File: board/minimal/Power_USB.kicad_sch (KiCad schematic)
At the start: 11 parts, among them J2 USB_C_Receptacle_USB2.0_14P, U4 STUSB4500QTR

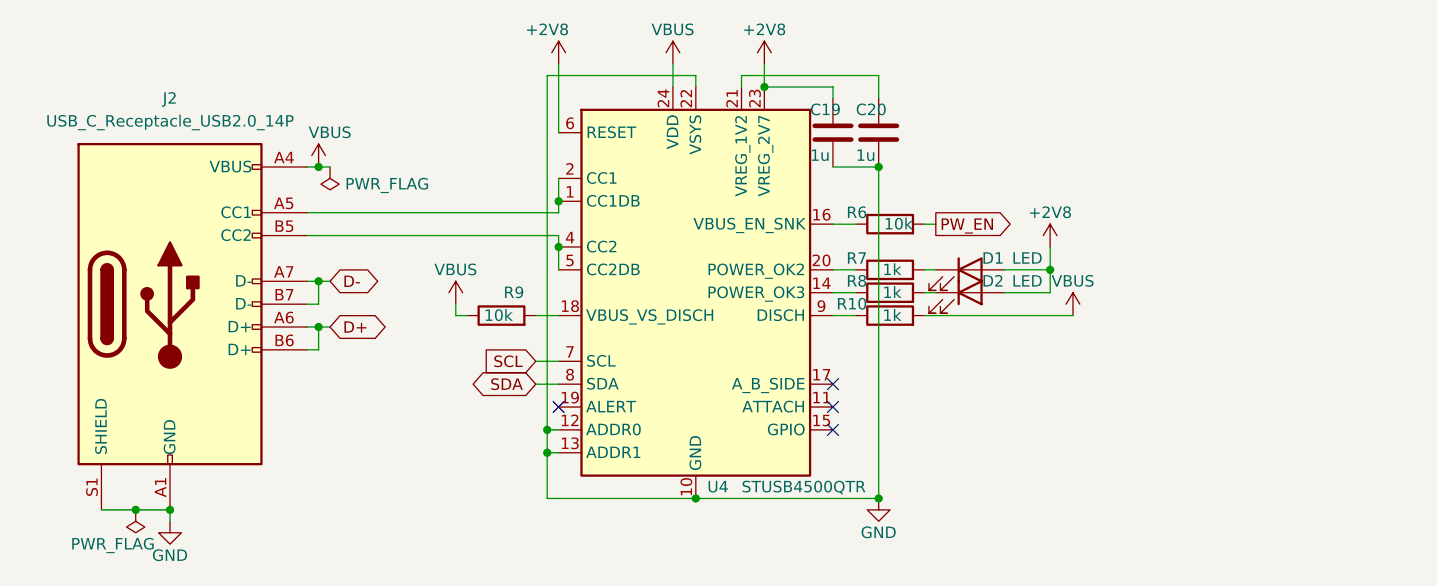
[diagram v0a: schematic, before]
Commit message: update PCB and edit schematic
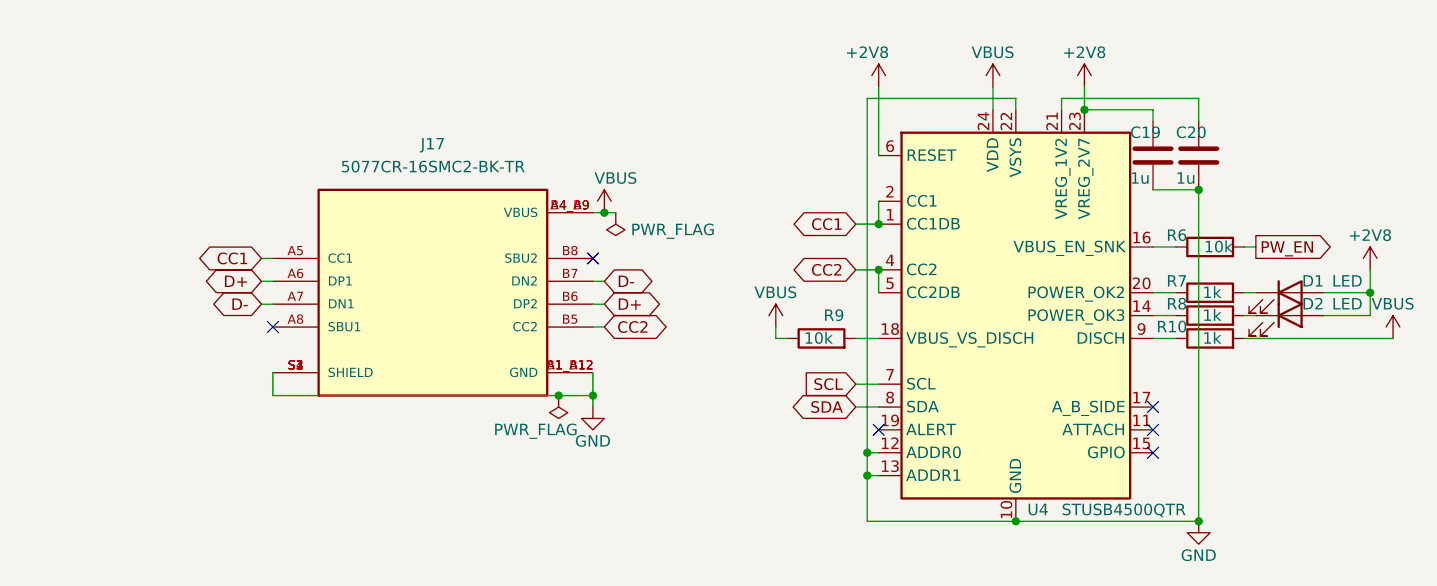
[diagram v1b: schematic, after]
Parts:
- removed J2: USB_C_Receptacle_USB2.0_14P, symbol Connector:USB_C_Receptacle_USB2.0_14P
- added J17: 5077CR-16SMC2-BK-TR, NELTRON_5077CR-16SMC2-BK-TR, symbol 5077CR-16SMC2-BK-TR:5077CR-16SMC2-BK-TR
- C19, C20: footprint (none) -> Capacitor_SMD:C_0603_1608Metric
- D1, D2: footprint (none) -> LED_SMD:LED_0603_1608Metric
- R10, R6, R7, R8, R9: footprint (none) -> Resistor_SMD:R_0603_1608Metric
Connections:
- net D+: now also J17.A6 (DP1), J17.B6 (DP2)
- net D-: now also J17.A7 (DN1), J17.B7 (DN2)
- net GND: now also J17.A1_B12 (GND), J17.B1_A12 (GND), J17.S1 (SHIELD), J17.S2 (SHIELD), J17.S3 (SHIELD), J17.S4 (SHIELD)
- net VBUS: now also J17.A4_B9 (VBUS), J17.B4_A9 (VBUS)
- net CC1: now reaches U4.1 (CC1DB), U4.2 (CC1)
- net CC1: now also J17.A5 (CC1)
- net CC2: now reaches U4.4 (CC2), U4.5 (CC2DB)
- net CC2: now also J17.B5 (CC2)
- no-connect marks 4 -> 6
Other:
- moved on the sheet: C19, C20, D1, D2, R10, R6, R7, R8, R9, U4
